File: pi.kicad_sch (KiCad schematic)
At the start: 4 parts, among them J5 2-1734839-5, U15 MCP23008-E/ML

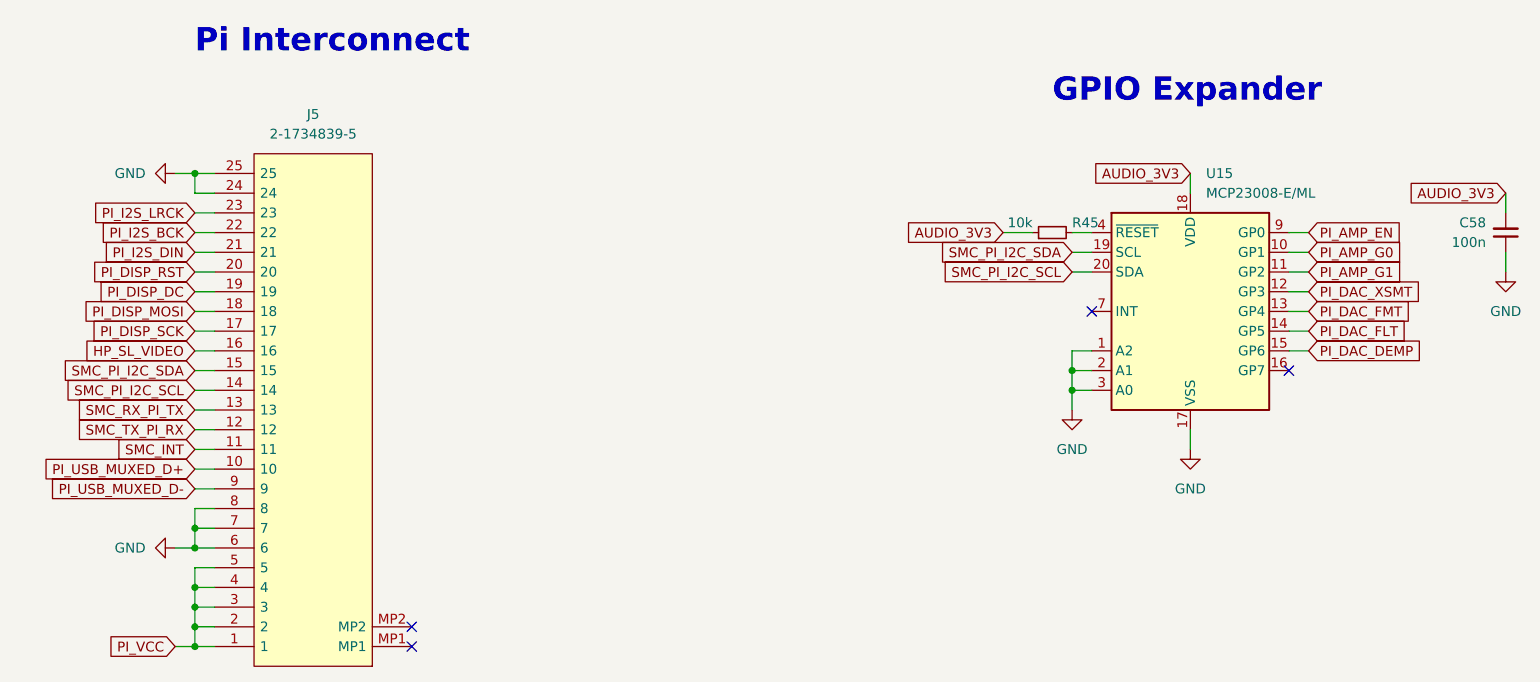
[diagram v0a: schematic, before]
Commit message: layout, routing: relayout and reroute board
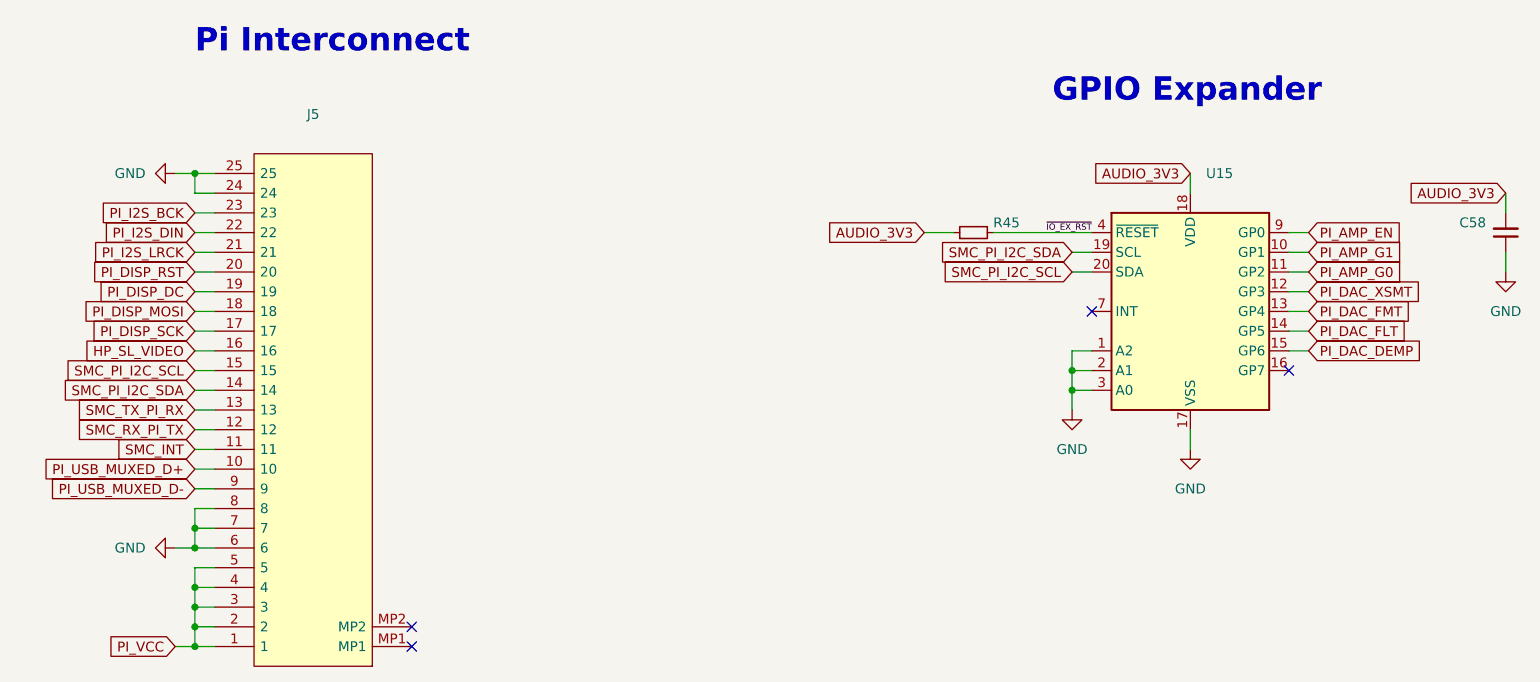
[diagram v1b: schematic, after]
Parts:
- C58: value 100n -> (none); footprint Capacitor_SMD:C_0402_1005Metric -> (none)
- J5: value 2-1734839-5 -> (none); footprint Gigahawk:217348395 -> (none)
- R45: value 10k -> (none); footprint Resistor_SMD:R_0402_1005Metric -> (none)
- U15: value MCP23008-E/ML -> (none); footprint Package_DFN_QFN:QFN-20-1EP_4x4mm_P0.5mm_EP2.7x2.7mm -> (none)
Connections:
- net PI_AMP_G0: now also U15.11 (GP2); no longer U15.10 (GP1)
- net PI_AMP_G1: now also U15.10 (GP1); no longer U15.11 (GP2)
- net PI_I2S_BCK: now also J5.23; no longer J5.22
- net PI_I2S_DIN: now also J5.22; no longer J5.21
- net PI_I2S_LRCK: now also J5.21; no longer J5.23
- net SMC_PI_I2C_SCL: now also J5.15; no longer J5.14
- net SMC_PI_I2C_SDA: now also J5.14; no longer J5.15
- net SMC_RX_PI_TX: now also J5.12; no longer J5.13
- net SMC_TX_PI_RX: now also J5.13; no longer J5.12
- net ~{IO_EX_RST}: now reaches R45.2, U15.4 (~{RESET})
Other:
- moved on the sheet: R45
